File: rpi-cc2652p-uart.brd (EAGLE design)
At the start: 46 x 20.5 mm, 13 parts, among them U1 CC2652P2-DUOWEISI, U2 AP2112K

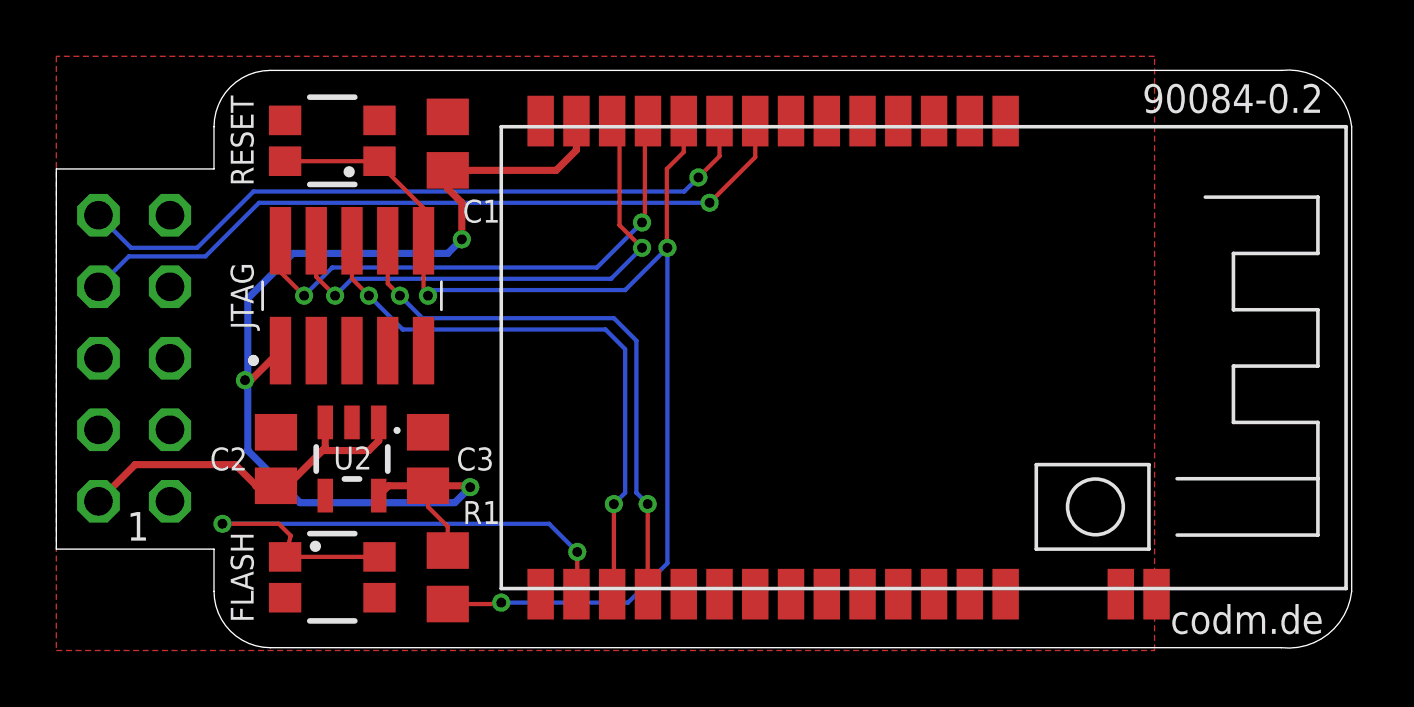
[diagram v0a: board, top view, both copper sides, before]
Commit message: bedder outline
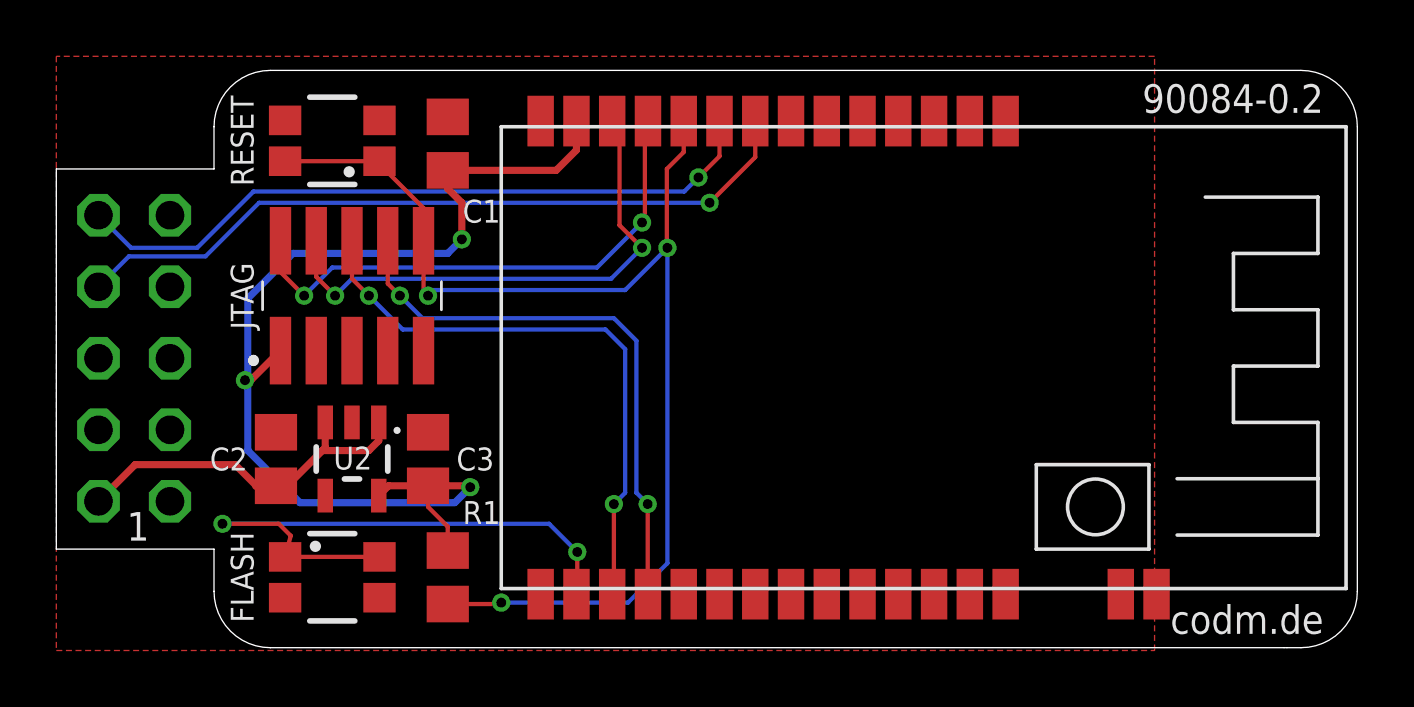
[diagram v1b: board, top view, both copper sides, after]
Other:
- board size 46 x 20.5 mm -> 46.2 x 20.5 mm
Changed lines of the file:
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@@
 <fusionsync huburn="a.cGVyc29uYWw6dWUyYzE1ODk4" projecturn="a.cGVyc29uYWw6dWUyYzE1ODk4IzIwMTkwNTIyMTk1MjcwNTc2" f3durn="urn:adsk.wipprod:dm.lineage:YxUaQjXaTCi4Y4MV4bwxpA" pcbguid="" lastpulledtime="" lastsyncedchangeguid="" latestrevisionid="9f82eda1-1b8b-46d7-8207-566304cbf3c7" lastsyncedrevisionid="9f82eda1-1b8b-46d7-8207-566304cbf3c7" lastboardhashguid="29e4727f-33c5-9ef5-bcef-569e12650b37" lastpushedtime="2021-04-15T11:45:35Z" linktopcb3d="true"/>
 <plain>
-<wire x1="7.6" y1="0" x2="43.5" y2="0" width="0" layer="20"/>
-<wire x1="46" y1="2" x2="46" y2="18.5" width="0" layer="20"/>
-<wire x1="43.5" y1="20.5" x2="7.6" y2="20.5" width="0" layer="20"/>
+<wire x1="7.6" y1="0" x2="43.6" y2="0" width="0" layer="20"/>
+<wire x1="43.6" y1="0" x2="43.7" y2="0" width="0" layer="20"/>
+<wire x1="46.2" y1="2" x2="46.2" y2="18.5" width="0" layer="20"/>
+<wire x1="44.2" y1="20.5" x2="7.6" y2="20.5" width="0" layer="20"/>
 <wire x1="7.6" y1="20.5" x2="5.6" y2="18.5" width="0" layer="20" curve="90"/>
 <wire x1="0" y1="17" x2="0" y2="3.5" width="0" layer="20"/>
@@
 <wire x1="5.6" y1="3.5" x2="5.6" y2="2" width="0" layer="20"/>
 <wire x1="5.6" y1="2" x2="7.6" y2="0" width="0" layer="20" curve="90"/>
-<wire x1="43.5" y1="0" x2="46" y2="2" width="0" layer="20" curve="90"/>
-<wire x1="46" y1="18.5" x2="43.5" y2="20.5" width="0" layer="20" curve="90"/>
 <text x="45.2" y="10.6" size="1.27" layer="26" rot="MR0">CC2652P2 RPi Serial
 ZigBee Module V0.2
@@
 <text x="45" y="19.5" size="1.016" layer="25" align="center-right">90084-0.2</text>
 <text x="45" y="1" size="1.016" layer="25" font="vector" align="center-right">codm.de</text>
+<wire x1="46.2" y1="18.5" x2="44.2" y2="20.5" width="0" layer="20" curve="90"/>
+<wire x1="46.2" y1="2" x2="44.2" y2="0" width="0" layer="20" curve="-90"/>
+<wire x1="44.2" y1="0" x2="43.7" y2="0" width="0" layer="20"/>
 </plain>
 <attributes>
